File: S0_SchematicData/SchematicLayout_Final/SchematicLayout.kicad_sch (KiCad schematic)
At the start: 9 parts, among them P1 Conn_Plug_2P, Q1 Q_NMOS, Q2 Q_NMOS, Q3 Q_NMOS, Q4 Q_NMOS, U1 LMZM23600V5, U2 ESP32-S2-WROVER

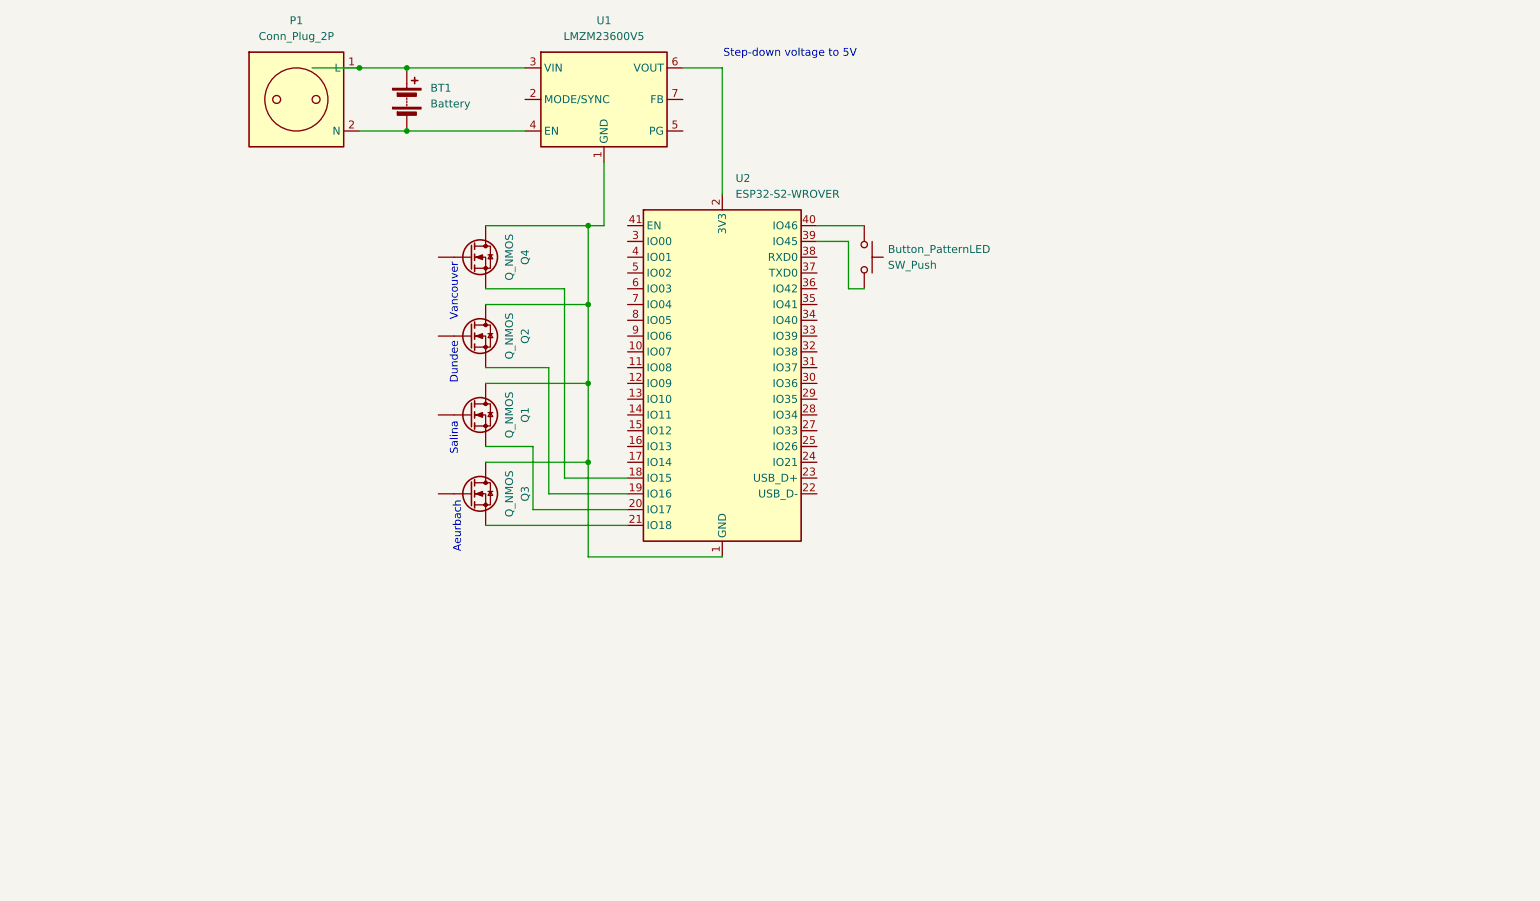
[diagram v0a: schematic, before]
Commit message: Sync and commit of current C code
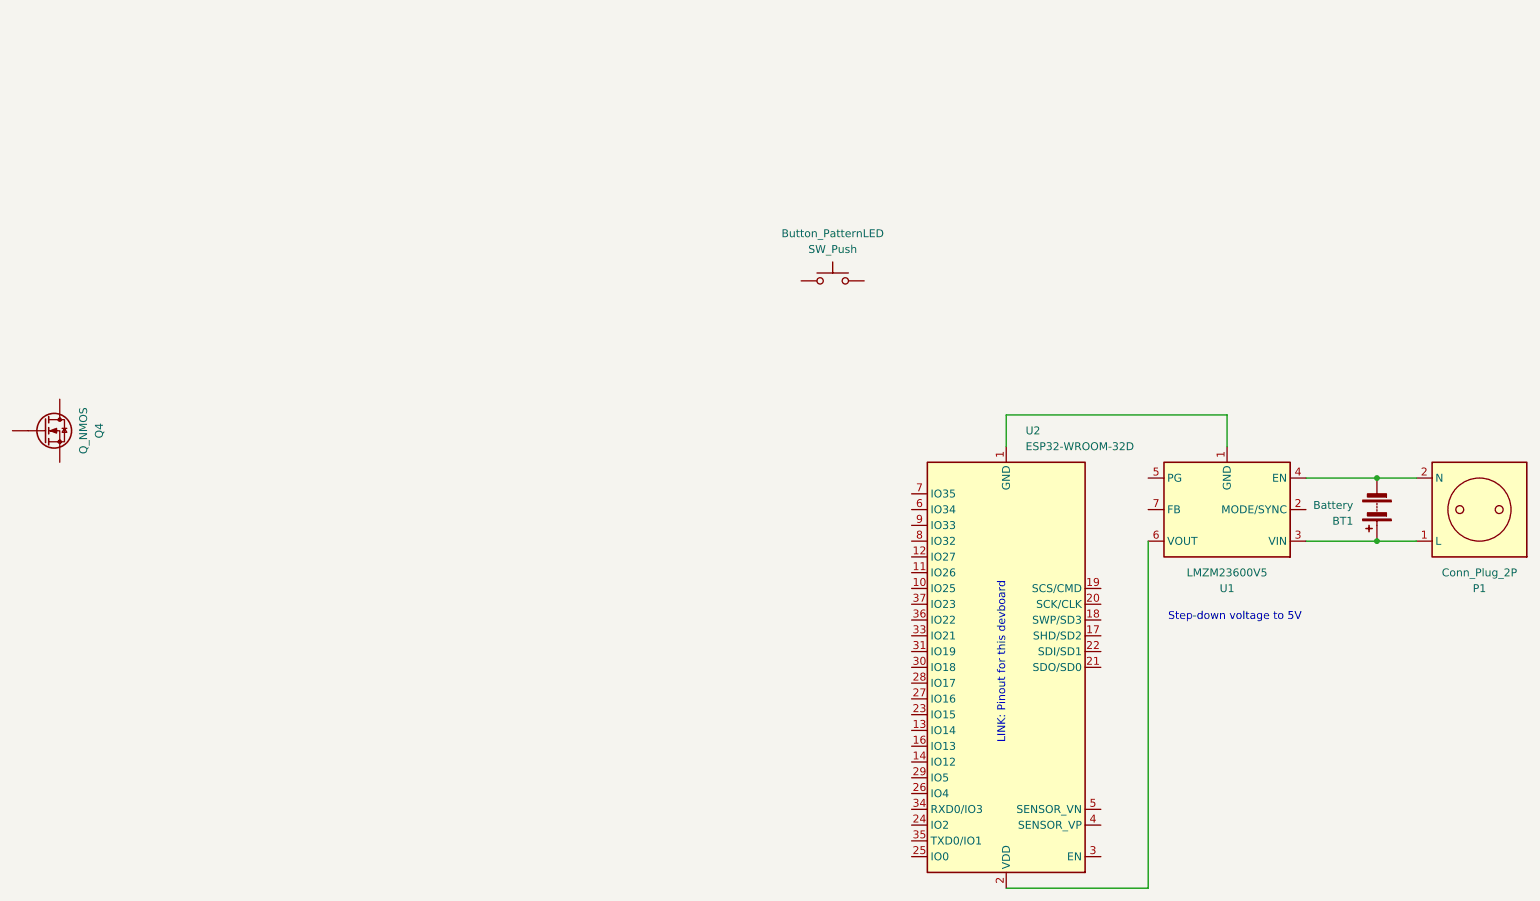
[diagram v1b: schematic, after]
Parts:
- removed Q1, Q2, Q3: Q_NMOS, symbol Device:Q_NMOS
- removed U2: ESP32-S2-WROVER, RF_Module:ESP32-S2-WROVER, symbol RF_Module:ESP32-S2-WROVER
- added U2: ESP32-WROOM-32D, RF_Module:ESP32-WROOM-32D, symbol RF_Module:ESP32-WROOM-32D
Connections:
- net at U1.1 (GND), U1.11 (GND): now also U2.1 (GND), U2.15 (GND), U2.38 (GND), U2.39 (GND); no longer Q4.D
- net at U1.6 (VOUT): now also U2.2 (VDD)
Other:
- note added: "LINK: Pinout for this devboard"
- note removed: "Aeurbach"
- note removed: "Dundee"
- note removed: "Salina"
- note removed: "Vancouver"
- moved on the sheet: BT1, Button_PatternLED, P1, Q4, U1
